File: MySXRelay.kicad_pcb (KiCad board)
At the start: 2 copper layers, 51 parts, among them K2 FH44L-1AT-L1-DC5V, Q1 2N7002, U1 MIC4427, U2 BL0942, U3 BP2525X, U4 Si8642BB-B-IS1, U5 MCP1703Ax-180xxTT

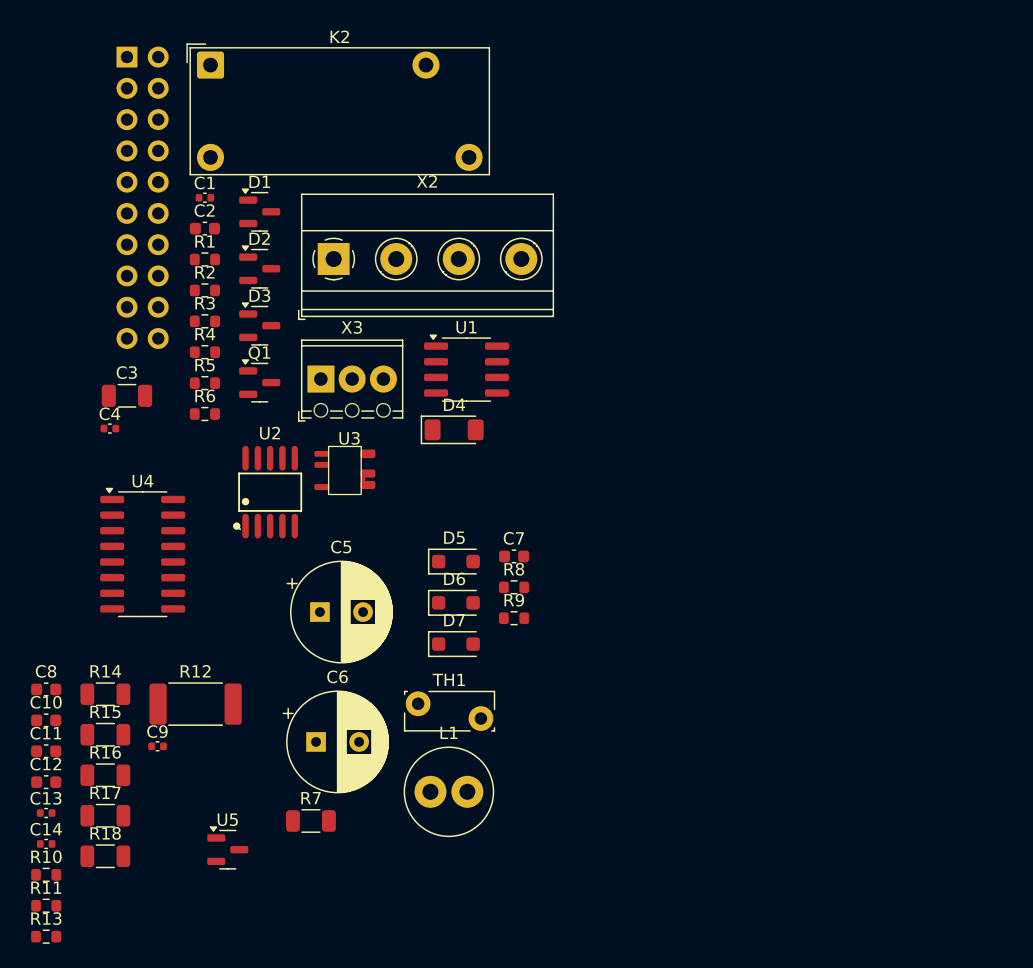
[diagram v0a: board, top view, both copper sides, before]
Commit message: setup PCS dimensions
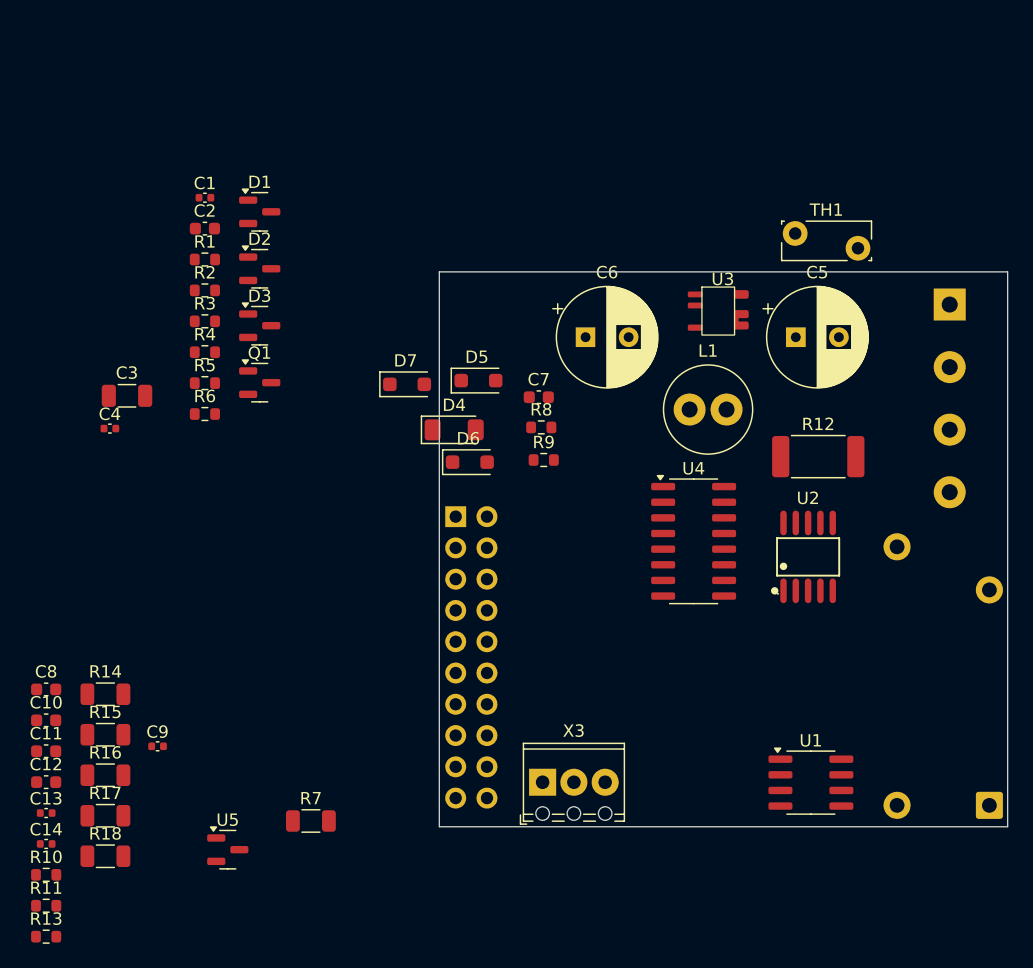
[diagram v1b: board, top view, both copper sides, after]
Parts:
- K2, X2: moved to B.Cu
- moved K2 87.3 mm to (180.1, 125.8), turned to 90 degrees
- moved R12 54.4 mm to (166.2, 97.5)
- moved X2 50.2 mm to (176.9, 85.1), turned to -90 degrees
- moved TH1 49.0 mm to (164.3, 79.3)
- moved X1 45.9 mm to (136.8, 102.3)
- moved U4 44.8 mm to (156.1, 104.4)
- moved C5 44.6 mm to (164.4, 87.8)
- moved U2 44.0 mm to (165.4, 105.6)
- moved U1 43.7 mm to (165.6, 124.0)
- moved C6 39.5 mm to (147.3, 87.8)
- moved L1 37.5 mm to (155.8, 93.7)
- moved X3 37.4 mm to (143.8, 123.9)
- moved U3 33.0 mm to (158.1, 85.5)
- moved D7 21.5 mm to (132.8, 91.6)
- moved D5 14.8 mm to (138.6, 91.3)
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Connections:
- X2 pad 1: L_OUT -> N_IN
- X2 pad 2: L_IN -> N_OUT
- X2 pad 3: N_OUT -> L_IN
- X2 pad 4: N_IN -> L_OUT
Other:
- board outline added: 46.2 x 45.1 mm
